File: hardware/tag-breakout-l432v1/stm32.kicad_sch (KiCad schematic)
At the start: 14 parts, among them J3 Conn_01x17, J4 Conn_01x17, J5 Conn_01x02_Male, Q1 Q_NPN_BEC, U3 stm32l432, U6 RV-3028-C7

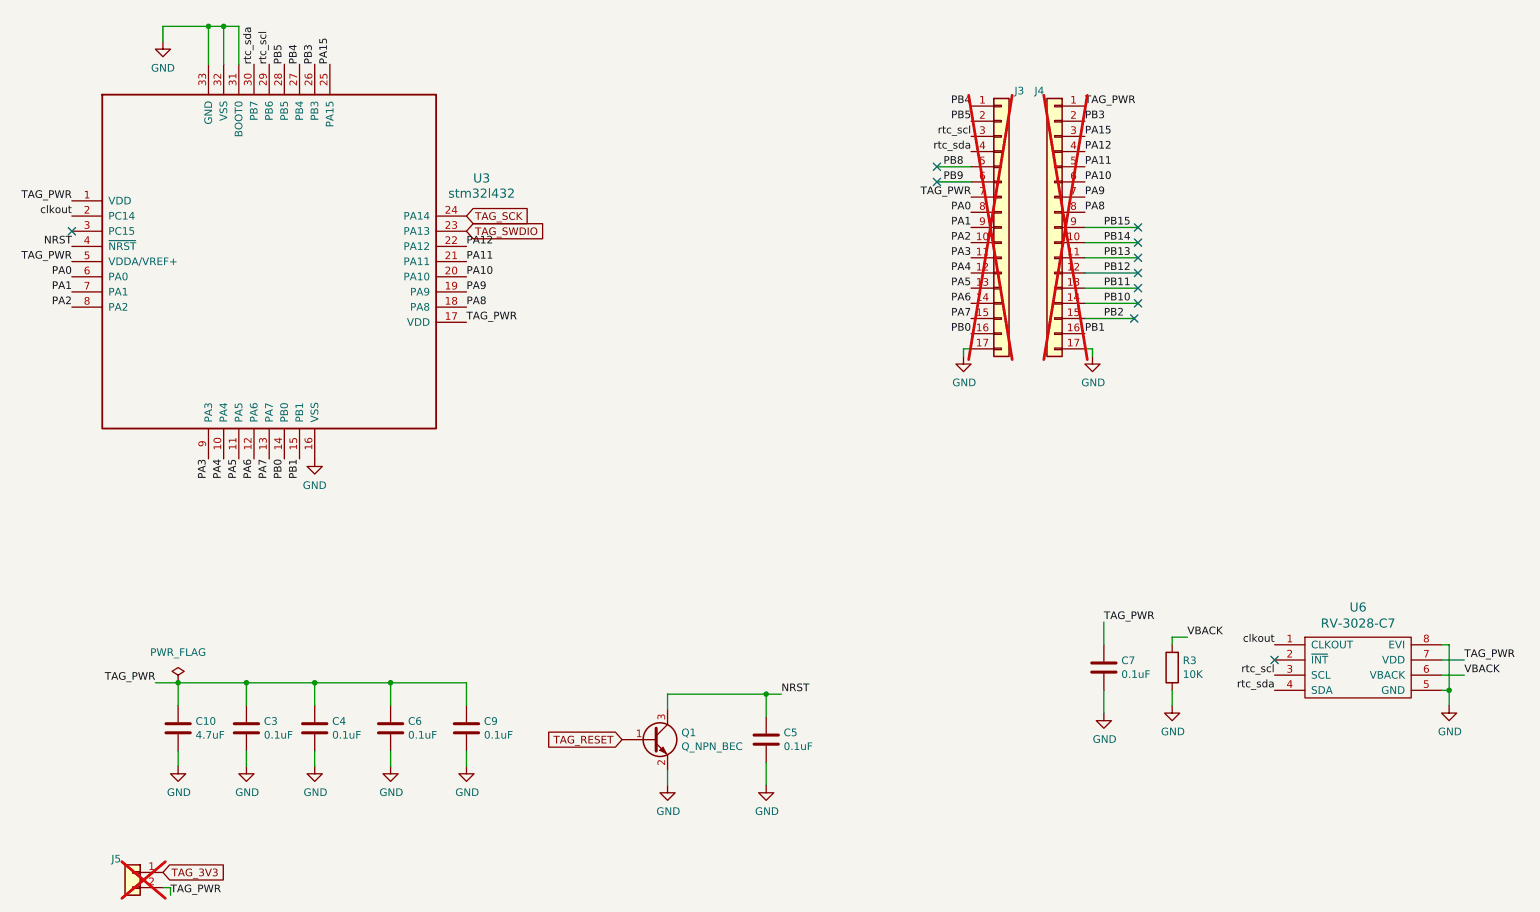
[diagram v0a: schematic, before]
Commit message: update proto boards
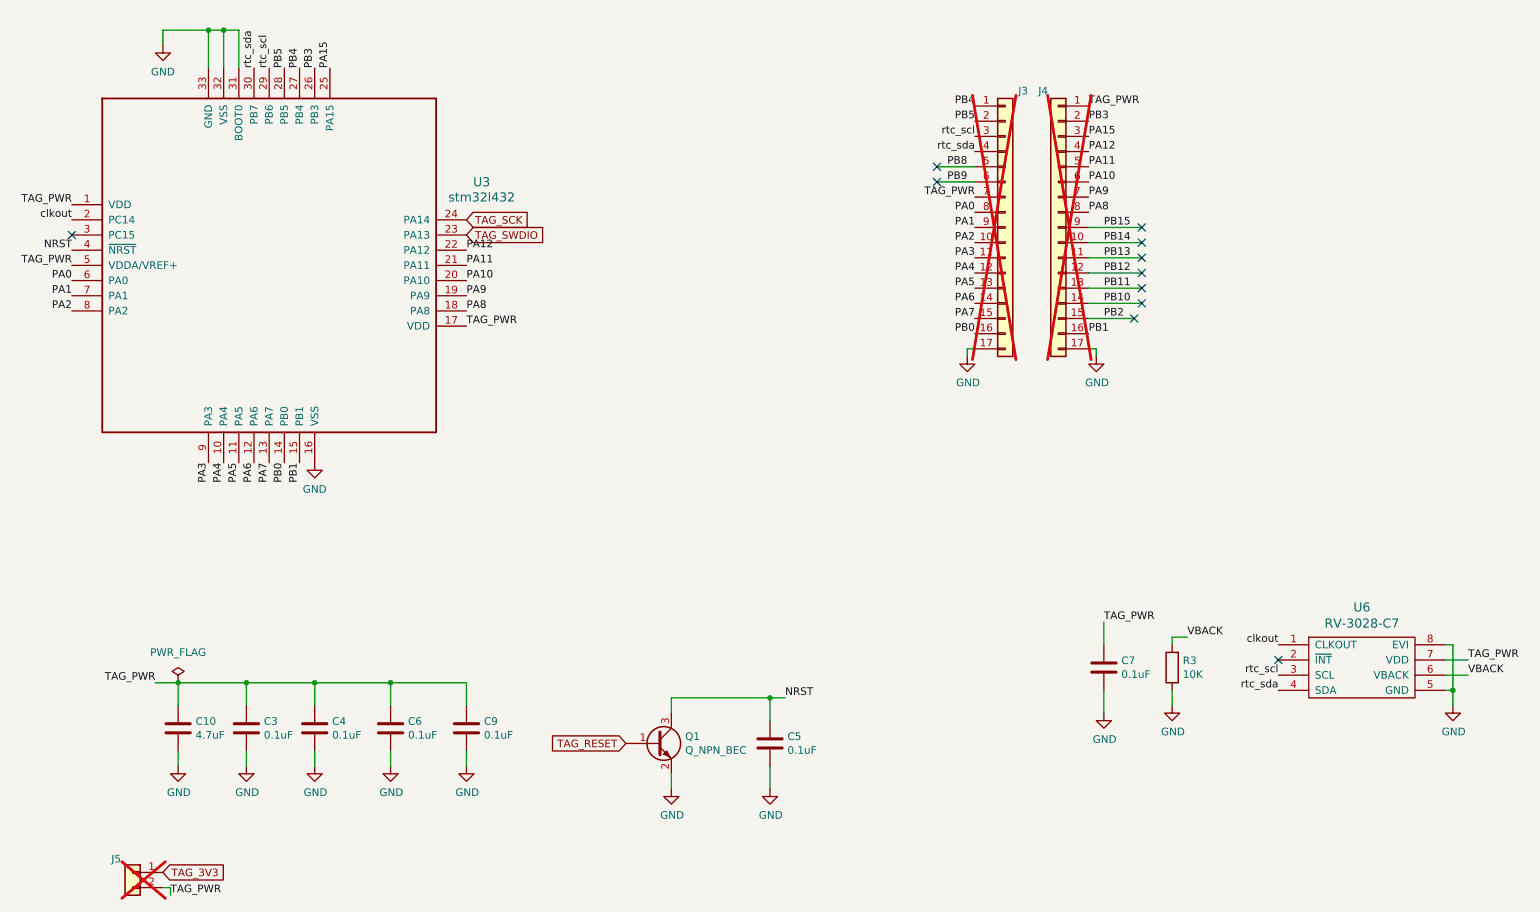
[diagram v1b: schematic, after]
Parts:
- J3, J4: footprint Connector_PinSocket_2.54mm:PinSocket_1x17_P2.54mm_Vertical -> library:PinHeader_1x17_P2.54mm_Vertical_Staggered
- U6: symbol tag-breakout-v2-rescue:RV-3028-C7-gpsparts -> tag-library:RV-3028-C7
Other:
- moved on the sheet: C5, J3, J4, Q1, U3, U6
